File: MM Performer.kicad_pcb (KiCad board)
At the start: 4 copper layers, 74.8 x 84.8 mm, 41 parts, among them IC1 68000D, J1 VCC, J2 GND, U1 MC68030RC, U2 MC68881FN-SOC, U3 ATF16V8BJ, U4 ATF16V8BJ, U5 ATF16V8BJ, U6 ATF16V8BJ, U7 ATF16V8BJ

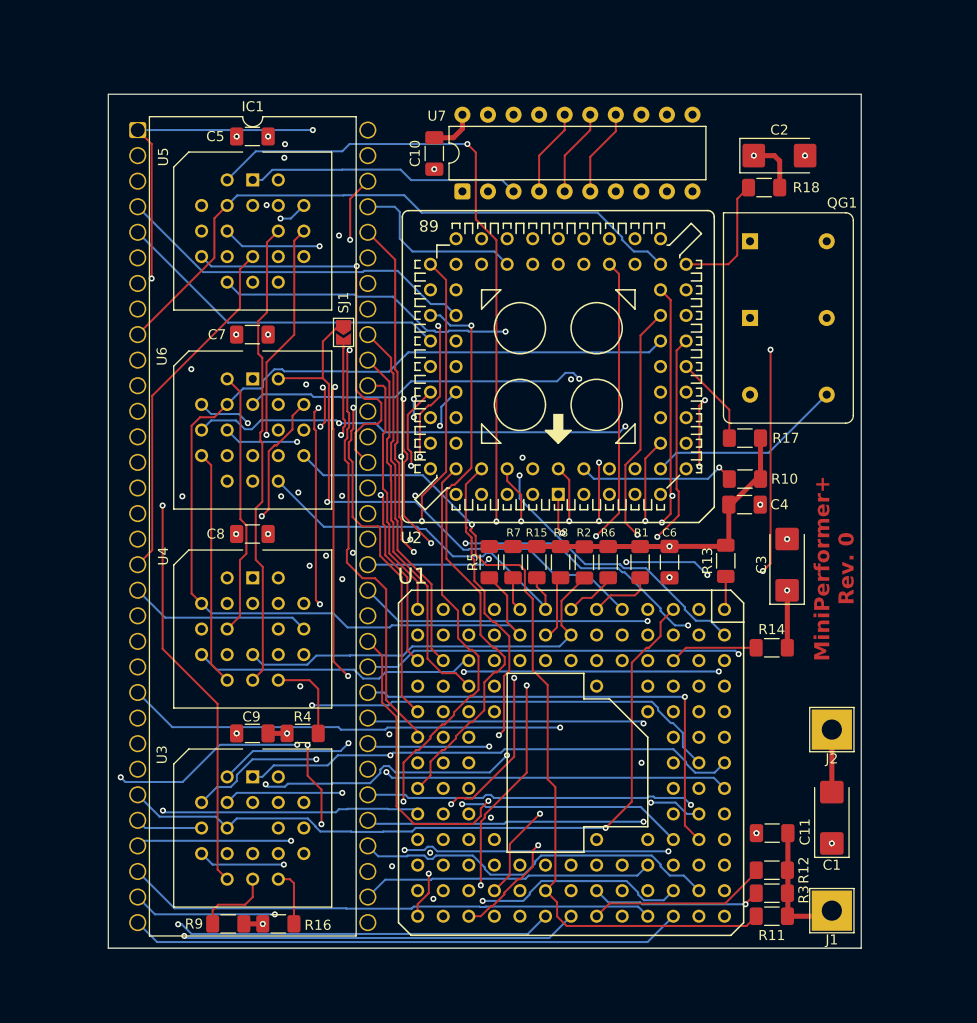
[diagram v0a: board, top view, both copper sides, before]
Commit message: Draw PCB
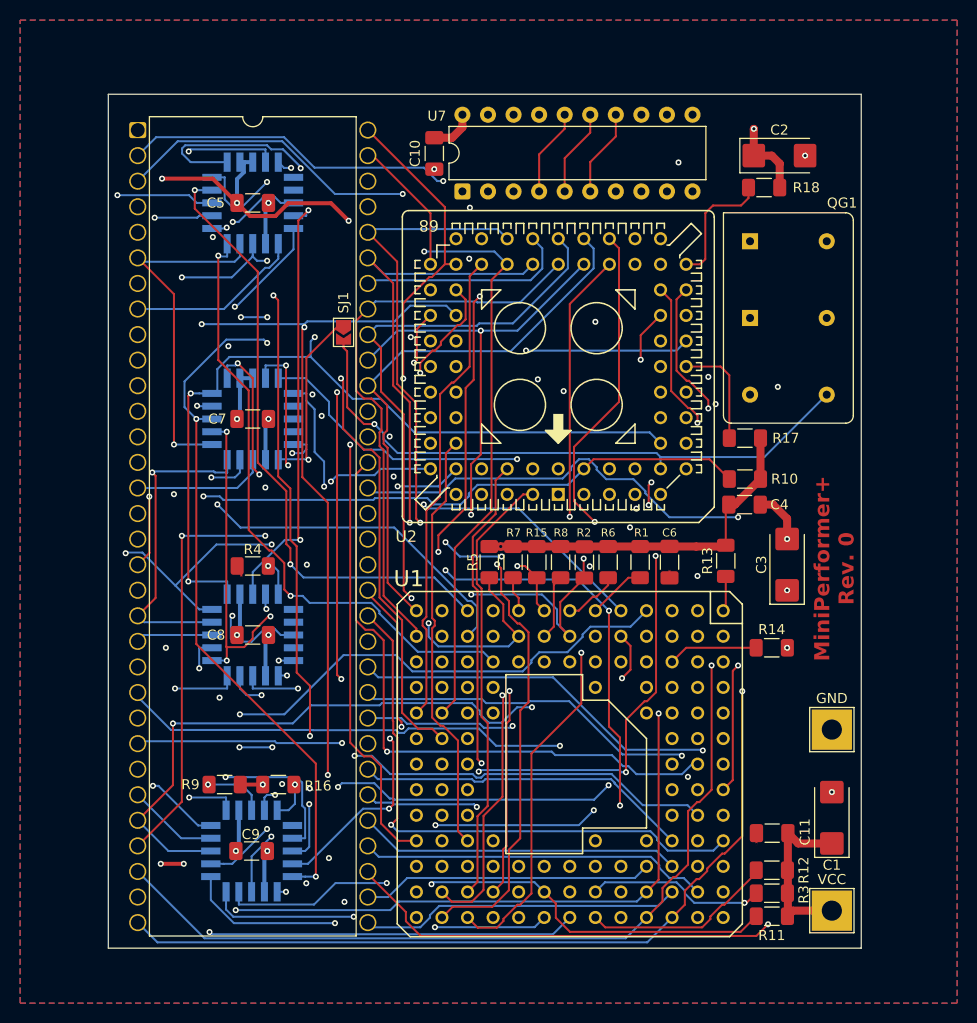
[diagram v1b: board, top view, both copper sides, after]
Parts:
- U3, U4, U5, U6: footprint footprints:PLCC-20_THT-Socket -> Package_LCC:PLCC-20_SMD-Socket; moved to B.Cu
- moved R4 17.4 mm to (50.2, 99.2)
- moved R9 13.8 mm to (47.4, 120.9)
- moved R16 13.8 mm to (52.7, 120.9)
- moved C9 11.7 mm to (50.0, 127.5)
- moved C8 10.0 mm to (50.2, 106.0)
- moved C7 8.38 mm to (50.2, 84.6)
- moved U3 7.37 mm to (50.0, 127.5)
- moved C5 6.60 mm to (50.2, 63.1)
- moved U4 5.67 mm to (50.2, 106.0)
- moved U6 3.98 mm to (50.2, 84.6)
- moved U5 2.29 mm to (50.2, 63.1)
- moved U1 0.18 mm to (81.7, 118.9)
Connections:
- U1 pad C5: (no net) -> GND
- U1 pad C6: (no net) -> VCC
- U1 pad C7: (no net) -> GND
- U1 pad C9: (no net) -> GND
- U1 pad D4: (no net) -> VCC
- U1 pad E3: (no net) -> GND
- U1 pad F2: (no net) -> VCC
- U1 pad F3: (no net) -> GND
- U1 pad G3: (no net) -> GND
- U1 pad H3: (no net) -> VCC
- U1 pad J3: (no net) -> GND
- U1 pad K4: (no net) -> VCC
- U1 pad L5: (no net) -> GND
- U1 pad L6: (no net) -> VCC
- U1 pad L7: (no net) -> GND
- U1 pad L8: (no net) -> GND
- U1 pad L9: (no net) -> GND
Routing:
- net GND: track 542.5 -> 659.5 mm, vias 10 -> 18
- net VCC: track 749.4 -> 654.6 mm, vias 9 -> 10
- net /A21: track 83.0 -> 128.4 mm, vias 2 -> 3
- net /A0: track 73.1 -> 105.2 mm, vias 2 -> 4
- net /D17: track 130.2 -> 99.5 mm, vias 2 -> 3
- net //R/W: track 127.4 -> 157.1 mm, vias 0 -> 5
- net /D20: track 127.8 -> 100.0 mm, vias 5 -> 2
- net /D7: track 44.1 -> 69.6 mm, vias 1 -> 3
- net /D14: track 68.6 -> 44.3 mm, vias 5 -> 0
- net /C8M.PDS: track 82.2 -> 105.5 mm, vias 0 -> 3
- net /N$1: track 13.2 -> 35.3 mm, vias 0 -> 3
- net /D16: track 119.8 -> 98.1 mm, vias 1 -> 4
- net //RESET_00: track 35.3 -> 53.8 mm, vias 0 -> 2
- net /A23: track 83.2 -> 101.5 mm, vias 1 -> 3
- net /D9: track 42.1 -> 59.9 mm, vias 1 -> 2
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- added copper zone on B.Cu, net GND
- added copper zone on F.Cu, net GND
- added copper zone on In1.Cu, net GND
- added copper zone on In2.Cu, net GND
